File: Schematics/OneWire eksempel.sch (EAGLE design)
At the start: 5 parts

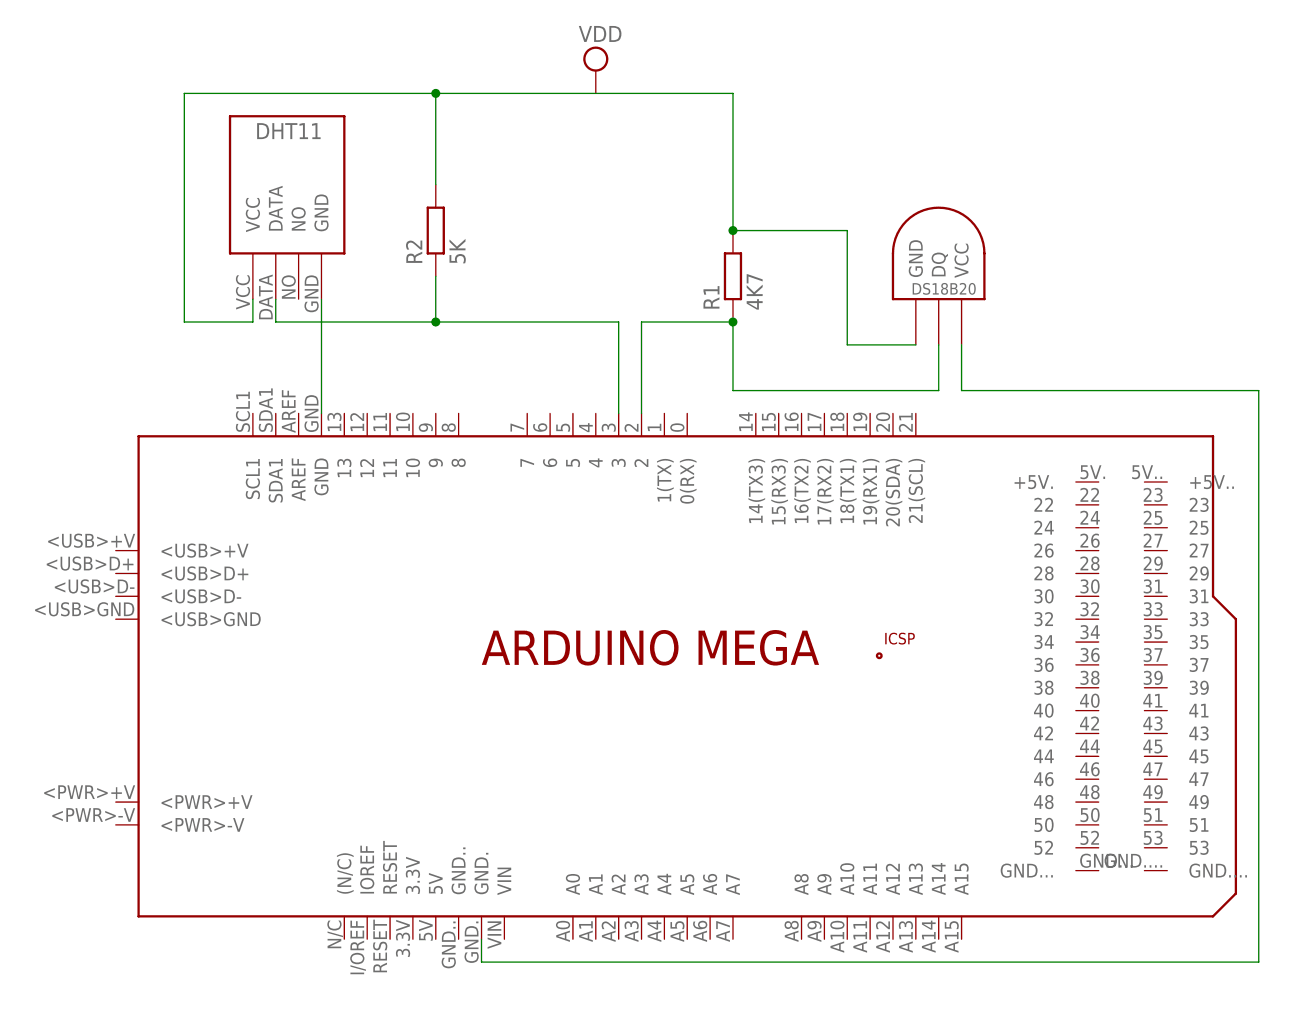
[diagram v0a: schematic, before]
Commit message: Onewire eksempel
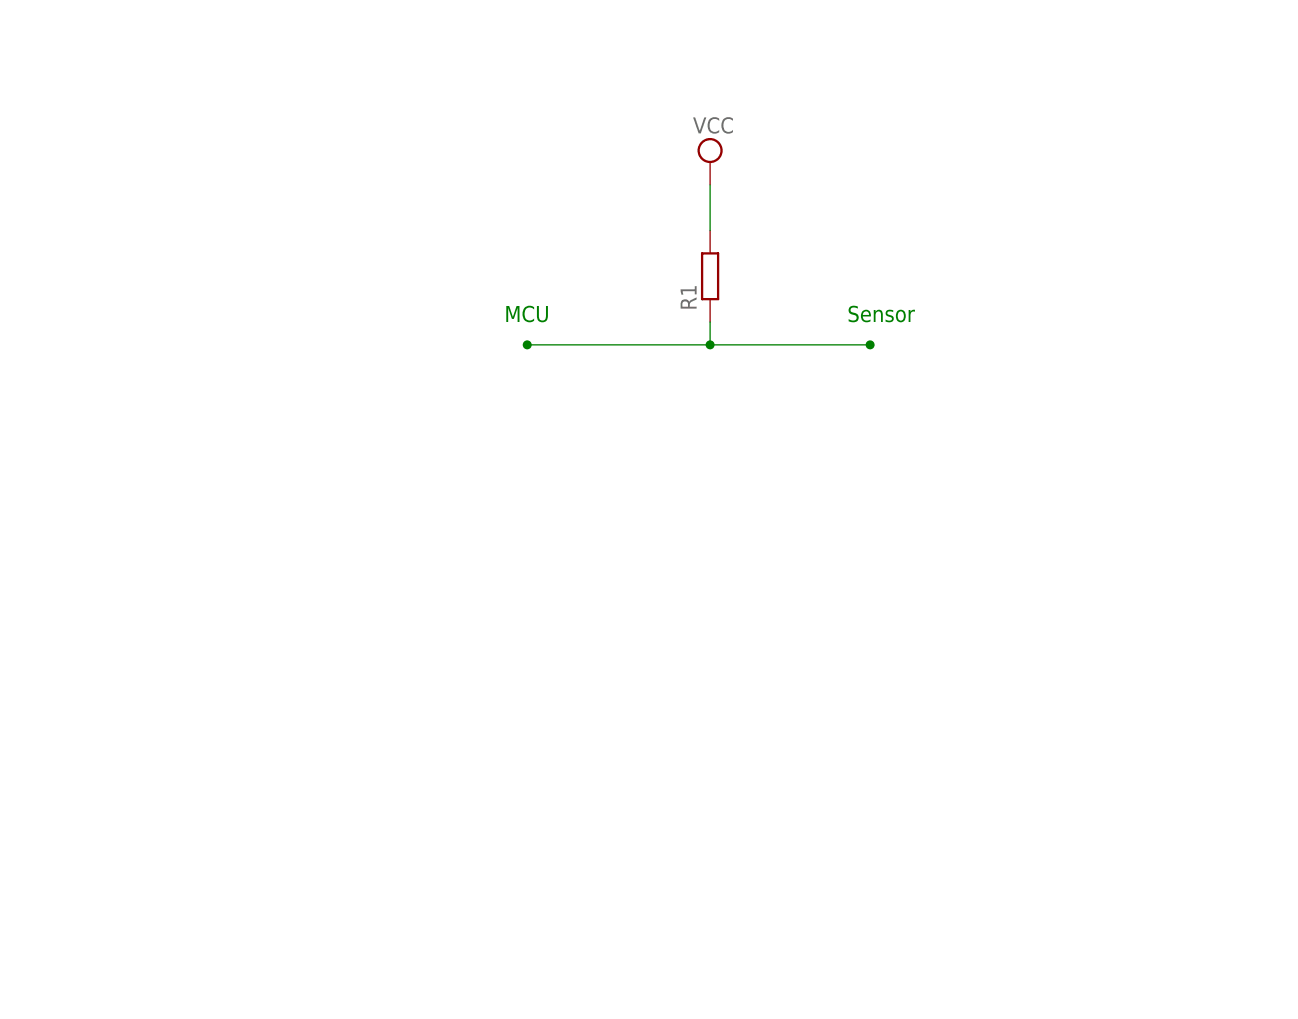
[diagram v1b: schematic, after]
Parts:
- removed PCB1: ARDUINO_MEGA, E14_Arduino:ARDUINO_MEGA
- removed R2: 5K, resistor:R-EU_0204/7
- removed U$1: DS1820TO92, Ava:DS1820TO92
- removed U$2: DHT11-PION., DHT11:DHT11-PION.
- R1: value 4K7 -> (none)
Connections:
- removed net N$2: PCB1.3, R2.1, U$2.DATA
- removed net N$3: PCB1.GND, U$2.GND
- removed net N$4: PCB1.GND., U$1.VCC
- removed net N$6: PCB1.2, R1.1, U$1.DQ
- removed net VDD: R1.2, R2.2, U$1.GND, U$2.VCC
- new net N$1: R1.1
- new net VCC: R1.2
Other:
- note added: "MCU"
- note added: "Sensor"
- moved on the sheet: R1
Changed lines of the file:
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@@
 <layer number="48" name="Document" color="7" fill="1" visible="no" active="no"/>
 <layer number="49" name="Reference" color="7" fill="1" visible="no" active="no"/>
-<layer number="50" name="dxf" color="7" fill="1" visible="no" active="no"/>
 <layer number="51" name="tDocu" color="7" fill="1" visible="no" active="no"/>
 <layer number="52" name="bDocu" color="7" fill="1" visible="no" active="no"/>
-<layer number="53" name="tGND_GNDA" color="7" fill="9" visible="no" active="no"/>
-<layer number="54" name="bGND_GNDA" color="1" fill="9" visible="no" active="no"/>
-<layer number="56" name="wert" color="7" fill="1" visible="no" active="no"/>
 <layer number="90" name="Modules" color="5" fill="1" visible="yes" active="yes"/>
 <layer number="91" name="Nets" color="2" fill="1" visible="yes" active="yes"/>
@@
 <layer number="98" name="Guide" color="6" fill="1" visible="yes" active="yes"/>
 <layer number="99" name="SpiceOrder" color="5" fill="1" visible="yes" active="yes"/>
-<layer number="100" name="Muster" color="7" fill="1" visible="no" active="no"/>
-<layer number="101" name="Patch_Top" color="12" fill="4" visible="no" active="yes"/>
-<layer number="102" name="Vscore" color="7" fill="1" visible="no" active="yes"/>
-<layer number="103" name="tMap" color="7" fill="1" visible="no" active="yes"/>
-<layer number="104" name="Name" color="7" fill="1" visible="no" active="yes"/>
-<layer number="105" name="tPlate" color="7" fill="1" visible="no" active="yes"/>
-<layer number="106" name="bPlate" color="7" fill="1" visible="no" active="yes"/>
-<layer number="107" name="Crop" color="7" fill="1" visible="no" active="yes"/>
-<layer number="116" name="Patch_BOT" color="9" fill="4" visible="no" active="yes"/>
-<layer number="121" name="_tsilk" color="7" fill="1" visible="no" active="yes"/>
-<layer number="122" name="_bsilk" color="7" fill="1" visible="no" active="yes"/>
-<layer number="125" name="_tNames" color="7" fill="1" visible="no" active="yes"/>
-<layer number="144" name="Drill_legend" color="7" fill="1" visible="no" active="yes"/>
-<layer number="151" name="HeatSink" color="7" fill="1" visible="no" active="yes"/>
-<layer number="200" name="200bmp" color="1" fill="10" visible="no" active="no"/>
-<layer number="201" name="201bmp" color="2" fill="1" visible="no" active="no"/>
-<layer number="202" name="202bmp" color="3" fill="1" visible="no" active="no"/>
-<layer number="203" name="203bmp" color="4" fill="10" visible="no" active="yes"/>
-<layer number="204" name="204bmp" color="5" fill="10" visible="no" active="yes"/>
-<layer number="205" name="205bmp" color="6" fill="10" visible="no" active="yes"/>
-<layer number="206" name="206bmp" color="7" fill="10" visible="no" active="yes"/>
-<layer number="207" name="207bmp" color="8" fill="10" visible="no" active="yes"/>
-<layer number="208" name="208bmp" color="9" fill="10" visible="no" active="yes"/>
-<layer number="209" name="209bmp" color="7" fill="1" visible="no" active="yes"/>
-<layer number="210" name="210bmp" color="7" fill="1" visible="no" active="yes"/>
-<layer number="211" name="211bmp" color="7" fill="1" visible="no" active="yes"/>
-<layer number="212" name="212bmp" color="7" fill="1" visible="no" active="yes"/>
-<layer number="213" name="213bmp" color="7" fill="1" visible="no" active="yes"/>
-<layer number="214" name="214bmp" color="7" fill="1" visible="no" active="yes"/>
-<layer number="215" name="215bmp" color="7" fill="1" visible="no" active="yes"/>
-<layer number="216" name="216bmp" color="7" fill="1" visible="no" active="yes"/>
-<layer number="217" name="217bmp" color="18" fill="1" visible="no" active="no"/>
-<layer number="218" name="218bmp" color="19" fill="1" visible="no" active="no"/>
-<layer number="219" name="219bmp" color="20" fill="1" visible="no" active="no"/>
-<layer number="220" name="220bmp" color="21" fill="1" visible="no" active="no"/>
-<layer number="221" name="221bmp" color="22" fill="1" visible="no" active="no"/>
-<layer number="222" name="222bmp" color="23" fill="1" visible="no" active="no"/>
-<layer number="223" name="223bmp" color="24" fill="1" visible="no" active="no"/>
-<layer number="224" name="224bmp" color="25" fill="1" visible="no" active="no"/>
-<layer number="250" name="Descript" color="3" fill="1" visible="no" active="no"/>
-<layer number="251" name="SMDround" color="12" fill="11" visible="no" active="no"/>
-<layer number="254" name="cooling" color="7" fill="1" visible="no" active="yes"/>
 </layers>
 <schematic xreflabel="%F%N/%S.%C%R" xrefpart="/%S.%C%R">
@@
 </classes>
 <parts>
-<part name="R1" library="resistor" deviceset="R-EU_" device="0204/7" value="4K7"/>
-<part name="ARDUINO5V" library="supply2" deviceset="VDD" device=""/>
-<part name="U$2" library="DHT11" deviceset="DHT11-PION." device=""/>
-<part name="R2" library="resistor" deviceset="R-EU_" device="0204/7" value="5K"/>
-<part name="PCB1" library="E14_Arduino" deviceset="ARDUINO_MEGA" device=""/>
-<part name="U$1" library="Ava" deviceset="DS1820" device="TO92"/>
+<part name="R1" library="resistor" deviceset="R-EU_" device="0204/7"/>
+<part name="SUPPLY1" library="supply2" deviceset="VCC" device=""/>
 </parts>
 <sheets>
 <sheet>
 <plain>
+<text x="7.62" y="50.8" size="1.778" layer="91">MCU</text>
+<text x="45.72" y="50.8" size="1.778" layer="91">Sensor</text>
 </plain>
 <instances>
-<instance part="R1" gate="G$1" x="33.02" y="55.88" rot="R90"/>
-<instance part="ARDUINO5V" gate="G$1" x="17.78" y="78.74"/>
-<instance part="U$2" gate="G$1" x="-17.78" y="66.04"/>
-<instance part="R2" gate="G$1" x="0" y="60.96" rot="R90"/>
-<instance part="PCB1" gate="G$1" x="25.4" y="12.7"/>
-<instance part="U$1" gate="G$1" x="55.88" y="53.34"/>
+<instance part="R1" gate="G$1" x="30.48" y="55.88" rot="R90"/>
+<instance part="SUPPLY1" gate="G$1" x="30.48" y="68.58"/>
 </instances>
 <busses>
 </busses>
 <nets>
-<net name="VDD" class="0">
+<net name="VCC" class="0">
 <segment>
-<pinref part="ARDUINO5V" gate="G$1" pin="VDD"/>
-<wire x1="17.78" y1="76.2" x2="0" y2="76.2" width="0.1524" layer="91"/>
-<wire x1="0" y1="76.2" x2="-27.94" y2="76.2" width="0.1524" layer="91"/>
-<wire x1="-27.94" y1="76.2" x2="-27.94" y2="50.8" width="0.1524" layer="91"/>
+<pinref part="SUPPLY1" gate="G$1" pin="VCC"/>
 <pinref part="R1" gate="G$1" pin="2"/>
-<wire x1="17.78" y1="76.2" x2="33.02" y2="76.2" width="0.1524" layer="91"/>
-<wire x1="33.02" y1="76.2" x2="33.02" y2="60.96" width="0.1524" layer="91"/>
-<pinref part="R2" gate="G$1" pin="2"/>
-<wire x1="0" y1="66.04" x2="0" y2="76.2" width="0.1524" layer="91"/>
-<junction x="0" y="76.2"/>
-<wire x1="45.72" y1="60.96" x2="33.02" y2="60.96" width="0.1524" layer="91"/>
-<junction x="33.02" y="60.96"/>
-<pinref part="U$2" gate="G$1" pin="VCC"/>
-<wire x1="-27.94" y1="50.8" x2="-20.32" y2="50.8" width="0.1524" layer="91"/>
-<wire x1="-20.32" y1="50.8" x2="-20.32" y2="53.34" width="0.1524" layer="91"/>
-<wire x1="45.72" y1="60.96" x2="45.72" y2="48.26" width="0.1524" layer="91"/>
-<pinref part="U$1" gate="G$1" pin="GND"/>
-<wire x1="45.72" y1="48.26" x2="53.34" y2="48.26" width="0.1524" layer="91"/>
+<wire x1="30.48" y1="66.04" x2="30.48" y2="60.96" width="0.1524" layer="91"/>
 </segment>
 </net>
-<net name="N$2" class="0">
+<net name="N$1" class="0">
 <segment>
-<pinref part="U$2" gate="G$1" pin="DATA"/>
-<wire x1="-17.78" y1="53.34" x2="-17.78" y2="50.8" width="0.1524" layer="91"/>
-<pinref part="PCB1" gate="G$1" pin="3"/>
-<wire x1="-17.78" y1="50.8" x2="0" y2="50.8" width="0.1524" layer="91"/>
-<wire x1="0" y1="50.8" x2="20.32" y2="50.8" width="0.1524" layer="91"/>
-<wire x1="20.32" y1="50.8" x2="20.32" y2="40.64" width="0.1524" layer="91"/>
-<pinref part="R2" gate="G$1" pin="1"/>
-<wire x1="0" y1="55.88" x2="0" y2="50.8" width="0.1524" layer="91"/>
-<junction x="0" y="50.8"/>
+<pinref part="R1" gate="G$1" pin="1"/>
+<wire x1="30.48" y1="50.8" x2="30.48" y2="48.26" width="0.1524" layer="91"/>
+<wire x1="10.16" y1="48.26" x2="30.48" y2="48.26" width="0.1524" layer="91"/>
+<wire x1="30.48" y1="48.26" x2="48.26" y2="48.26" width="0.1524" layer="91"/>
+<junction x="30.48" y="48.26"/>
+<junction x="10.16" y="48.26"/>
+<junction x="48.26" y="48.26"/>
 </segment>
 </net>
-<net name="N$4" class="0">
-<segment>
-<pinref part="U$1" gate="G$1" pin="VCC"/>
-<wire x1="58.42" y1="43.18" x2="58.42" y2="48.26" width="0.1524" layer="91"/>
-<wire x1="58.42" y1="43.18" x2="91.44" y2="43.18" width="0.1524" layer="91"/>
-<wire x1="91.44" y1="43.18" x2="91.44" y2="-20.32" width="0.1524" layer="91"/>
-<pinref part="PCB1" gate="G$1" pin="GND."/>
-<wire x1="91.44" y1="-20.32" x2="5.08" y2="-20.32" width="0.1524" layer="91"/>
-<wire x1="5.08" y1="-20.32" x2="5.08" y2="-17.78" width="0.1524" layer="91"/>
-</segment>
-</net>
-<net name="N$3" class="0">
-<segment>
-<pinref part="PCB1" gate="G$1" pin="GND"/>
-<wire x1="-12.7" y1="53.34" x2="-12.7" y2="40.64" width="0.1524" layer="91"/>
-<pinref part="U$2" gate="G$1" pin="GND"/>
-</segment>
-</net>
-<net name="N$6" class="0">
-<segment>
-<wire x1="22.86" y1="50.8" x2="22.86" y2="40.64" width="0.1524" layer="91"/>
-<pinref part="PCB1" gate="G$1" pin="2"/>
-<pinref part="R1" gate="G$1" pin="1"/>
-<wire x1="33.02" y1="43.18" x2="33.02" y2="50.8" width="0.1524" layer="91"/>
-<wire x1="22.86" y1="50.8" x2="33.02" y2="50.8" width="0.1524" layer="91"/>
-<junction x="33.02" y="50.8"/>
-<pinref part="U$1" gate="G$1" pin="DQ"/>
-<wire x1="33.02" y1="43.18" x2="55.88" y2="43.18" width="0.1524" layer="91"/>
-<wire x1="55.88" y1="43.18" x2="55.88" y2="48.26" width="0.1524" layer="91"/>
-</segment>
-</net>
